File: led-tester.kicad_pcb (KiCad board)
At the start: 2 copper layers, 50 x 50 mm, 30 parts, among them J1 PWR, J2 PWR, J3 VOLT, J4 LED, SW1 LED_POL, SW2 1mA, SW3 2mA, SW4 3mA, SW5 5mA, SW6 10mA, SW7 20mA, U1 PAM2804, U2 LM321

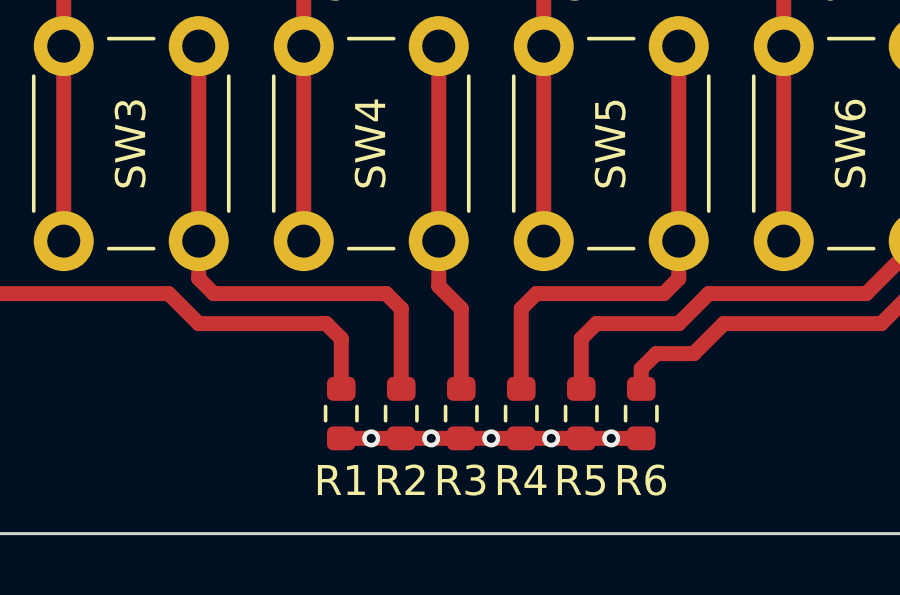
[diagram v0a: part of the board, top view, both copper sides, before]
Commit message: Final tweaks and bom
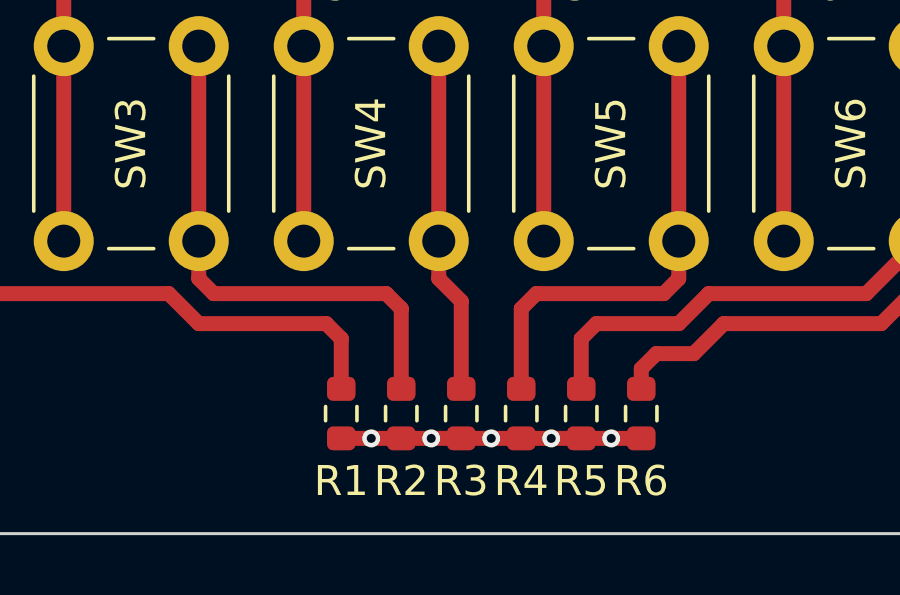
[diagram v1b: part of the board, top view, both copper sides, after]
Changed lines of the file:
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@@
   (net 14 "Net-(R2-Pad1)")
   (net 15 "Net-(R3-Pad1)")
-  (net 16 "Net-(SW5-Pad2)")
-  (net 17 "Net-(SW6-Pad2)")
-  (net 18 "Net-(SW7-Pad2)")
+  (net 16 "Net-(R4-Pad1)")
+  (net 17 "Net-(R5-Pad1)")
+  (net 18 "Net-(R6-Pad1)")
   (net 19 "Net-(J4-Pad1)")
   (net 20 "Net-(J4-Pad10)")
@@
       (net 6 "LED-") (pinfunction "1") (pintype "passive"))
     (pad "2" thru_hole circle (at 6.5 4.5 180) (size 2 2) (drill 1.1) (layers *.Cu *.Mask)
-      (net 16 "Net-(SW5-Pad2)") (pinfunction "2") (pintype "passive"))
+      (net 16 "Net-(R4-Pad1)") (pinfunction "2") (pintype "passive"))
     (pad "2" thru_hole circle (at 0 4.5 180) (size 2 2) (drill 1.1) (layers *.Cu *.Mask)
-      (net 16 "Net-(SW5-Pad2)") (pinfunction "2") (pintype "passive"))
+      (net 16 "Net-(R4-Pad1)") (pinfunction "2") (pintype "passive"))
     (model "${KICAD6_3DMODEL_DIR}/Button_Switch_THT.3dshapes/SW_PUSH_6mm_H8mm.wrl"
       (offset (xyz 0 0 0))
@@
       (net 6 "LED-") (pinfunction "1") (pintype "passive"))
     (pad "2" thru_hole circle (at 6.5 4.5 180) (size 2 2) (drill 1.1) (layers *.Cu *.Mask)
-      (net 17 "Net-(SW6-Pad2)") (pinfunction "2") (pintype "passive"))
+      (net 17 "Net-(R5-Pad1)") (pinfunction "2") (pintype "passive"))
     (pad "2" thru_hole circle (at 0 4.5 180) (size 2 2) (drill 1.1) (layers *.Cu *.Mask)
-      (net 17 "Net-(SW6-Pad2)") (pinfunction "2") (pintype "passive"))
+      (net 17 "Net-(R5-Pad1)") (pinfunction "2") (pintype "passive"))
     (model "${KICAD6_3DMODEL_DIR}/Button_Switch_THT.3dshapes/SW_PUSH_6mm_H8mm.wrl"
       (offset (xyz 0 0 0))
@@
     (fp_line (start 0.8 0.4125) (end -0.8 0.4125) (layer "F.Fab") (width 0.1))
     (pad "1" smd roundrect (at -0.825 0 270) (size 0.8 0.95) (layers "F.Cu" "F.Paste" "F.Mask") (roundrect_rratio 0.25)
-      (net 18 "Net-(SW7-Pad2)") (pintype "passive"))
+      (net 18 "Net-(R6-Pad1)") (pintype "passive"))
     (pad "2" smd roundrect (at 0.825 0 270) (size 0.8 0.95) (layers "F.Cu" "F.Paste" "F.Mask") (roundrect_rratio 0.25)
       (net 2 "GND") (pintype "passive"))
@@
     (fp_line (start -0.8 0.4125) (end -0.8 -0.4125) (layer "F.Fab") (width 0.1))
     (pad "1" smd roundrect (at -0.825 0 270) (size 0.8 0.95) (layers "F.Cu" "F.Paste" "F.Mask") (roundrect_rratio 0.25)
-      (net 17 "Net-(SW6-Pad2)") (pintype "passive"))
+      (net 17 "Net-(R5-Pad1)") (pintype "passive"))
     (pad "2" smd roundrect (at 0.825 0 270) (size 0.8 0.95) (layers "F.Cu" "F.Paste" "F.Mask") (roundrect_rratio 0.25)
       (net 2 "GND") (pintype "passive"))
@@
       (net 6 "LED-") (pinfunction "1") (pintype "passive"))
     (pad "2" thru_hole circle (at 0 4.5 180) (size 2 2) (drill 1.1) (layers *.Cu *.Mask)
-      (net 18 "Net-(SW7-Pad2)") (pinfunction "2") (pintype "passive"))
+      (net 18 "Net-(R6-Pad1)") (pinfunction "2") (pintype "passive"))
     (pad "2" thru_hole circle (at 6.5 4.5 180) (size 2 2) (drill 1.1) (layers *.Cu *.Mask)
-      (net 18 "Net-(SW7-Pad2)") (pinfunction "2") (pintype "passive"))
+      (net 18 "Net-(R6-Pad1)") (pinfunction "2") (pintype "passive"))
     (model "${KICAD6_3DMODEL_DIR}/Button_Switch_THT.3dshapes/SW_PUSH_6mm_H8mm.wrl"
       (offset (xyz 0 0 0))
@@
     (fp_line (start -0.8 0.4125) (end -0.8 -0.4125) (layer "F.Fab") (width 0.1))
     (pad "1" smd roundrect (at -0.825 0 270) (size 0.8 0.95) (layers "F.Cu" "F.Paste" "F.Mask") (roundrect_rratio 0.25)
-      (net 16 "Net-(SW5-Pad2)") (pintype "passive"))
+      (net 16 "Net-(R4-Pad1)") (pintype "passive"))
     (pad "2" smd roundrect (at 0.825 0 270) (size 0.8 0.95) (layers "F.Cu" "F.Paste" "F.Mask") (roundrect_rratio 0.25)
       (net 2 "GND") (pintype "passive"))
@@
   (segment (start 115.75 92) (end 115.25 91.5) (width 0.5) (layer "F.Cu") (net 14))
   (segment (start 123.25 83.75) (end 123.25 90.25) (width 0.5) (layer "F.Cu") (net 15))
-  (segment (start 124 92.5) (end 124 95.175) (width 0.5) (layer "F.Cu") (net 15))
-  (segment (start 123.25 91.75) (end 124 92.5) (width 0.5) (layer "F.Cu") (net 15))
-  (segment (start 123.25 90.25) (end 123.25 91.75) (width 0.5) (layer "F.Cu") (net 15))
+  (segment (start 123.25 91.5) (end 124 92.25) (width 0.5) (layer "F.Cu") (net 15))
+  (segment (start 124 92.25) (end 124 95.175) (width 0.5) (layer "F.Cu") (net 15))
+  (segment (start 123.25 90.25) (end 123.25 91.5) (width 0.5) (layer "F.Cu") (net 15))
   (segment (start 130.75 92) (end 126.5 92) (width 0.5) (layer "F.Cu") (net 16))
   (segment (start 131.25 83.75) (end 131.25 90.25) (width 0.5) (layer "F.Cu") (net 16))
